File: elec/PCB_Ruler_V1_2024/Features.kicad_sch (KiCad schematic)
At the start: 0 parts

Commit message: IMU
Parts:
- added C1, C2, C3: 1uF, symbol Device:C
- added MT1: ICM-42670-P, IMU:XDCR_ICM-42670-P, symbol ICM-42670-P:ICM-42670-P
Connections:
- new net +3.3V: C1.1, C2.1, C3.1, MT1.5 (VDDIO), MT1.8 (VDD)
- new net GND: C1.2, C2.2, C3.2

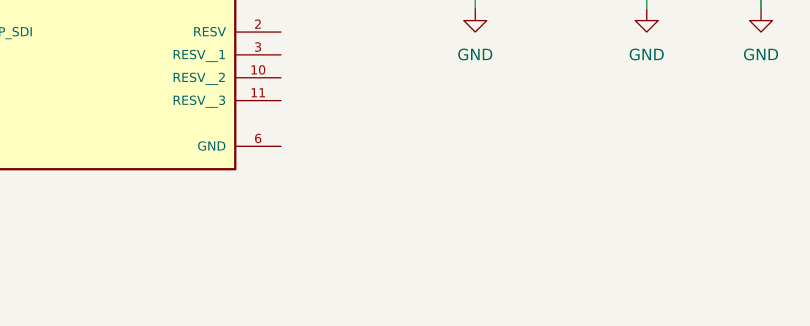
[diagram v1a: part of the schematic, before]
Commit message: battery charger
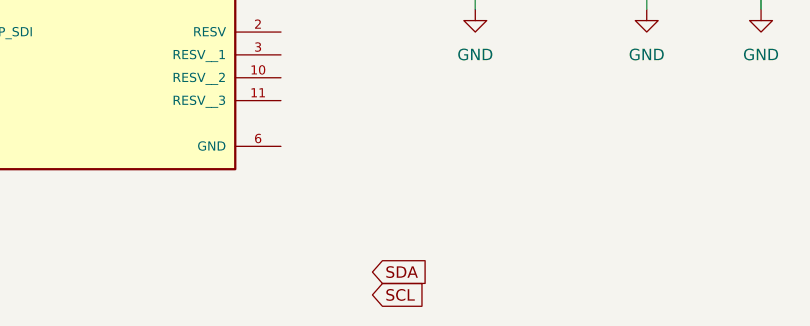
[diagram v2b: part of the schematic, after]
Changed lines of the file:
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@@
+		)
+	)
+	(global_label "SDA"
+		(shape input)
+		(at 113.03 99.06 0)
+		(fields_autoplaced yes)
+		(effects
+			(font
+				(size 1.27 1.27)
+			)
+			(justify left)
+		)
+		(property "Intersheetrefs" "${INTERSHEET_REFS}"
+			(at 119.5833 99.06 0)
+			(effects
+				(font
+					(size 1.27 1.27)
+				)
+				(justify left)
+				(hide yes)
+			)
+		)
+	)
+	(global_label "SCL"
+		(shape input)
+		(at 113.03 101.6 0)
+		(fields_autoplaced yes)
+		(effects
+			(font
+				(size 1.27 1.27)
+			)
+			(justify left)
+		)
+		(property "Intersheetrefs" "${INTERSHEET_REFS}"
+			(at 119.5228 101.6 0)
+			(effects
+				(font
+					(size 1.27 1.27)
+				)
+				(justify left)
+				(hide yes)
+			)
 		)
 	)
@@
 		)
 		(instances
-			(project ""
+			(project "PCB_Ruler_V1_2024"
 				(path "/e39575e5-bba1-47dc-9ccf-32a84e6da237/ca7d0597-655a-4aee-bb72-0094cc7418df"
 					(reference "MT1")
@@
 		)
 		(instances
-			(project ""
+			(project "PCB_Ruler_V1_2024"
 				(path "/e39575e5-bba1-47dc-9ccf-32a84e6da237/ca7d0597-655a-4aee-bb72-0094cc7418df"
 					(reference "#PWR04")
@@
 		)
 		(instances
-			(project ""
+			(project "PCB_Ruler_V1_2024"
 				(path "/e39575e5-bba1-47dc-9ccf-32a84e6da237/ca7d0597-655a-4aee-bb72-0094cc7418df"
 					(reference "C1")
@@
 		)
 		(instances
-			(project ""
+			(project "PCB_Ruler_V1_2024"
 				(path "/e39575e5-bba1-47dc-9ccf-32a84e6da237/ca7d0597-655a-4aee-bb72-0094cc7418df"
 					(reference "#PWR02")
